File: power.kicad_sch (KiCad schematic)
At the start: 13 parts, among them U2 AP2112K-3.3

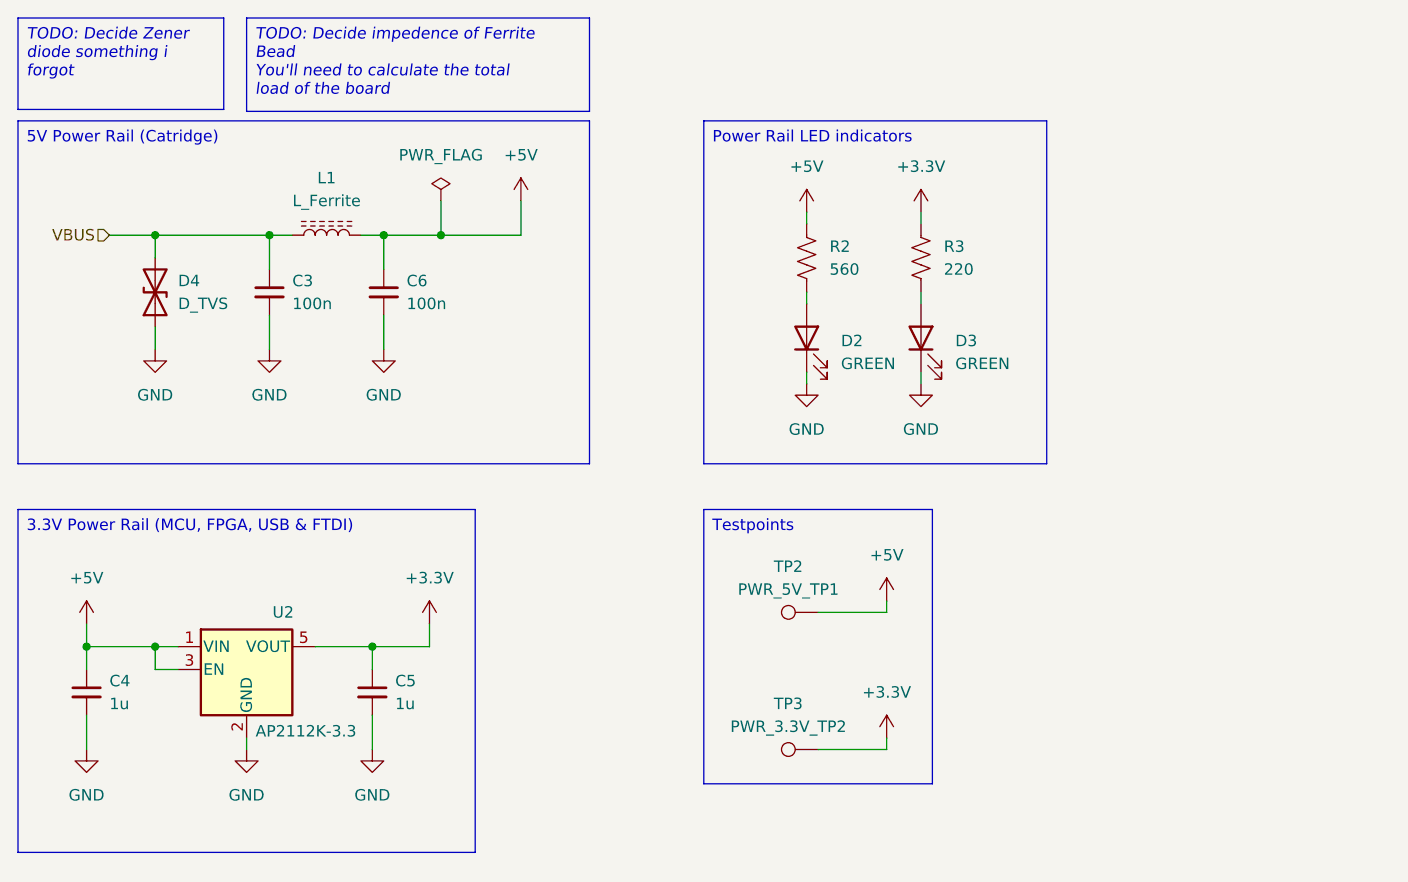
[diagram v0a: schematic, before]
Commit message: Power rail stuff
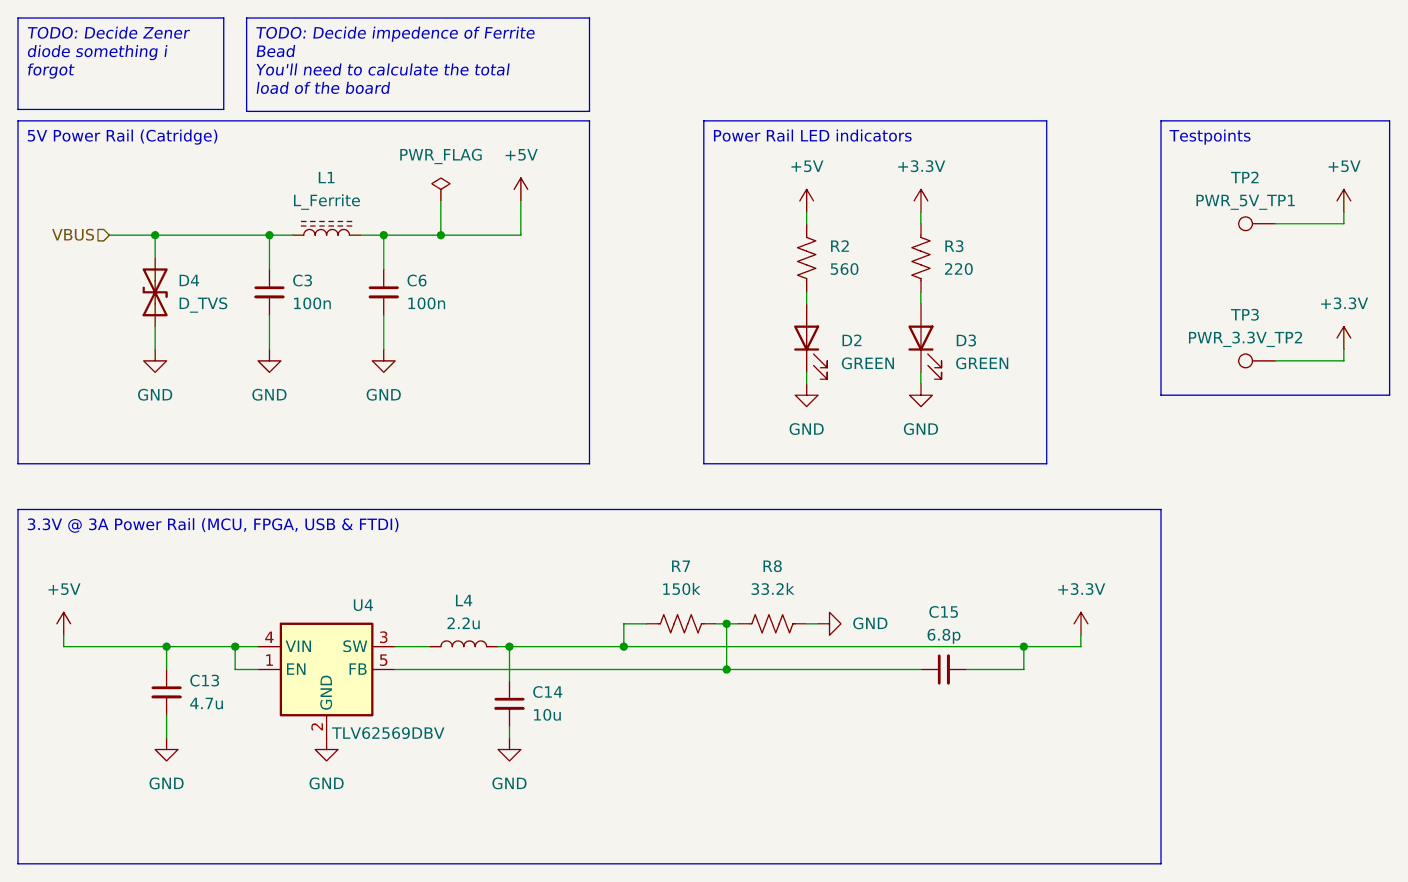
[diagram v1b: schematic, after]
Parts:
- removed C4, C5: 1u, symbol Device:C_Small
- removed U2: AP2112K-3.3, Package_TO_SOT_SMD:SOT-23-5, symbol Regulator_Linear:AP2112K-3.3
- added C13: 4.7u, symbol Device:C_Small
- added C14: 10u, symbol Device:C_Small
- added C15: 6.8p, symbol Device:C_Small
- added L4: 2.2u, symbol Device:L
- added R7: 150k, symbol Device:R_US
- added R8: 33.2k, symbol Device:R_US
- added U4: TLV62569DBV, Package_TO_SOT_SMD:SOT-23-5, symbol Regulator_Switching:TLV62569DBV
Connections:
- net +3.3V: now also C14.1, C15.2, L4.2, R7.1
- net +5V: now also C13.1, U4.1 (EN), U4.4 (VIN)
- net GND: now also C13.2, C14.2, R8.2, U4.2 (GND)
- new net: C15.1, R7.2, R8.1, U4.5 (FB)
- new net: L4.1, U4.3 (SW)
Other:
- moved on the sheet: TP2, TP3
